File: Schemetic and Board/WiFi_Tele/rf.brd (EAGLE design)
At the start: 57.9 x 33.3 mm, 22 parts

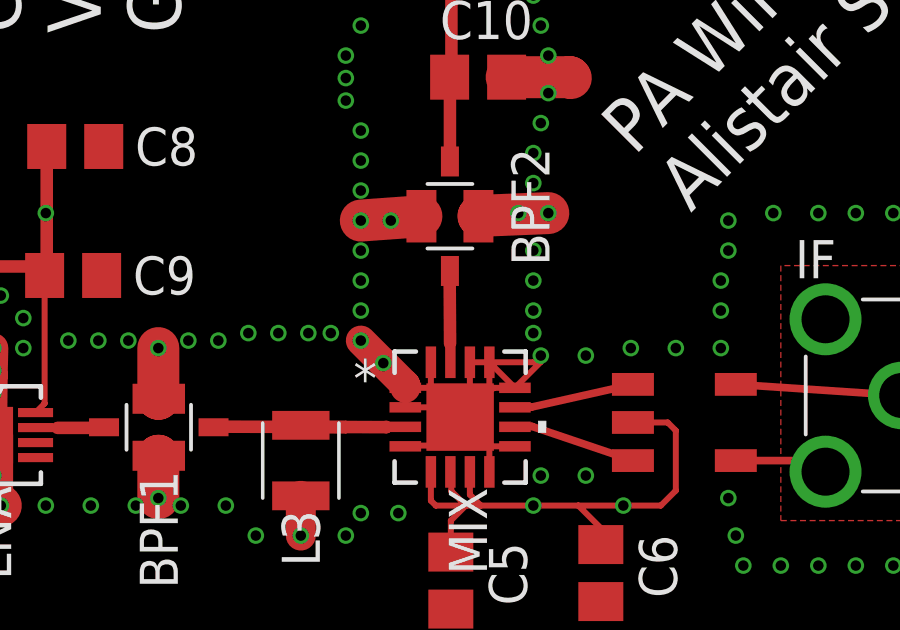
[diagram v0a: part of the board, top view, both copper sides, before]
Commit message: Deleted a whole bunch of stuff which shouldn't be in the repo
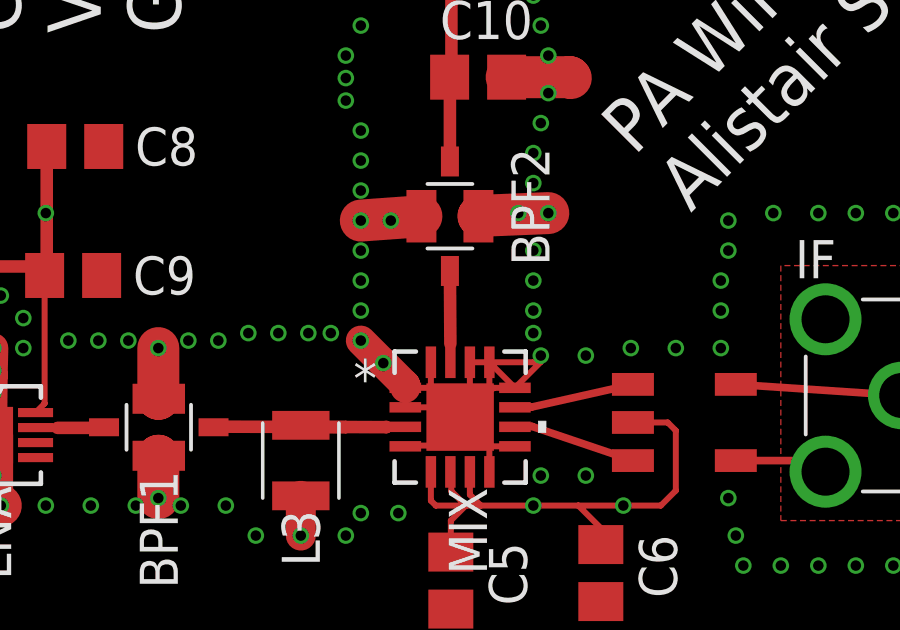
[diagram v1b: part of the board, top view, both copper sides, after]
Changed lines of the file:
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@@
 <?xml version="1.0" encoding="utf-8"?>
 <!DOCTYPE eagle SYSTEM "eagle.dtd">
-<eagle version="9.1.2">
+<eagle version="9.1.3">
 <drawing>
 <settings>
-<setting alwaysvectorfont="yes"/>
+<setting alwaysvectorfont="no"/>
 <setting verticaltext="up"/>
 </settings>
@@
 </polygon>
 <contactref element="LNA" pad="9"/>
-<polygon width="0.127" layer="1" rank="6">
+<polygon width="0.127" layer="1" isolate="0.254" rank="6">
 <vertex x="0.5" y="40"/>
 <vertex x="0.5" y="7.5"/>
@@
 <contactref element="BPF2" pad="I/O$2"/>
 <contactref element="MIX" pad="15"/>
-<wire x1="35.975" y1="18.287396875" x2="35.975" y2="18.9" width="0.2032" layer="1"/>
-<wire x1="35.975" y1="18.9" x2="35.9600625" y2="21.3100625" width="0.41896875" layer="1"/>
-<wire x1="35.9600625" y1="21.3100625" x2="35.97" y2="21.32" width="0.41896875" layer="1"/>
-<wire x1="35.985" y1="18.277396875" x2="35.975" y2="18.287396875" width="0.2032" layer="1"/>
+<wire x1="35.985" y1="18.277396875" x2="35.985" y2="18.89" width="0.2032" layer="1"/>
+<wire x1="35.985" y1="18.89" x2="35.969940625" y2="21.32" width="0.41896875" layer="1"/>
+<wire x1="35.970184375" y1="21.32" x2="35.97" y2="21.32" width="0.41896875" layer="1"/>
+<wire x1="35.970184375" y1="21.32" x2="35.969940625" y2="21.32" width="0.41896875" layer="1"/>
 </signal>
 <signal name="5V">
